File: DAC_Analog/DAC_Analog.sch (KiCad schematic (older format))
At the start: 17 parts, among them J1 SPDIF_RX_1, J2 SPDIF_RX_2, J3 SPDIF_RX_3, J4 SPDIF_RX_4, J5 I2C_IN, J6 OutR, J7 OutL, J8 Alim_DAC, J9 Alim_SRC, U1 ISO154x

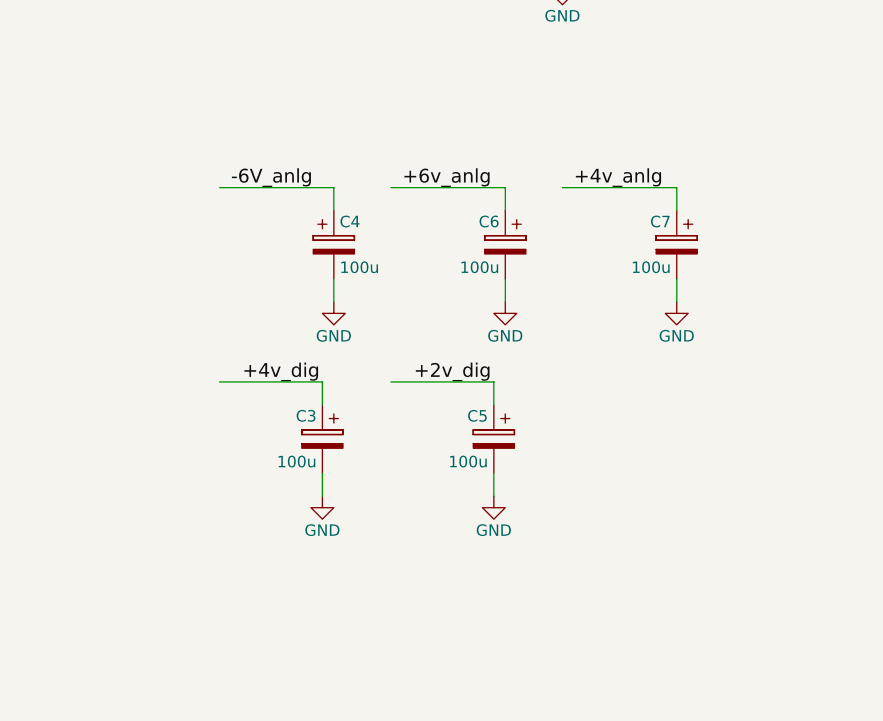
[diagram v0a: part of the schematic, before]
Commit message: Update layout
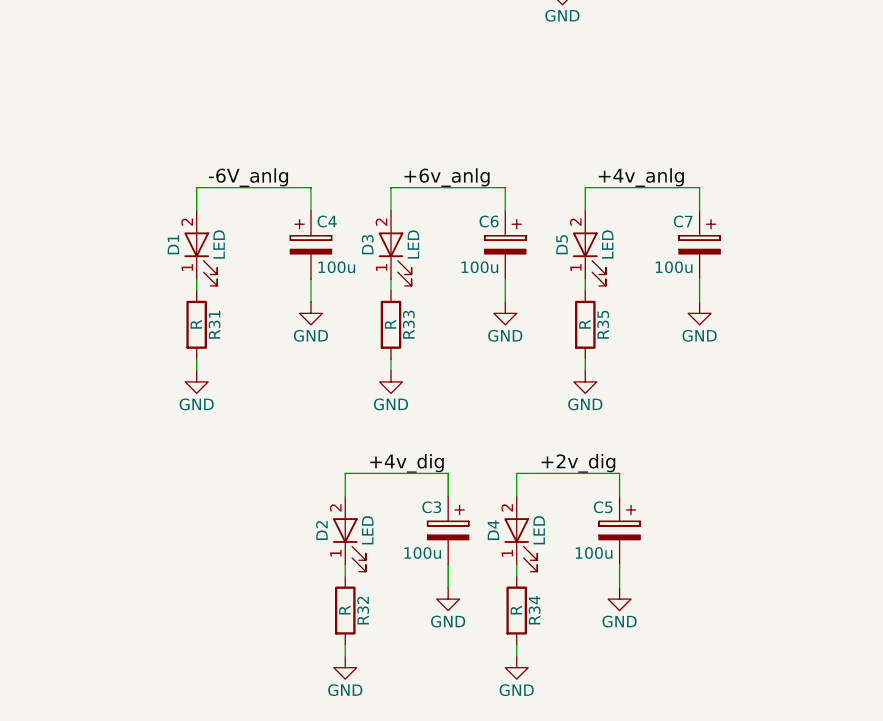
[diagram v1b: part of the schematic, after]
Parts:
- added D1, D2, D3, D4, D5: LED, Yame_library:SM0603-LED-MR, symbol LED
- added R31, R32, R33, R34, R35: R, Yame_library:SM0603-MR, symbol R
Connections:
- wire segments 91 -> 106
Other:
- moved on the sheet: C3, C4, C5, C7
